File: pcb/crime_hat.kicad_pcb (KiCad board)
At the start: 2 copper layers, 3 parts, among them Q1 2N2222, Q2 FQP27P06

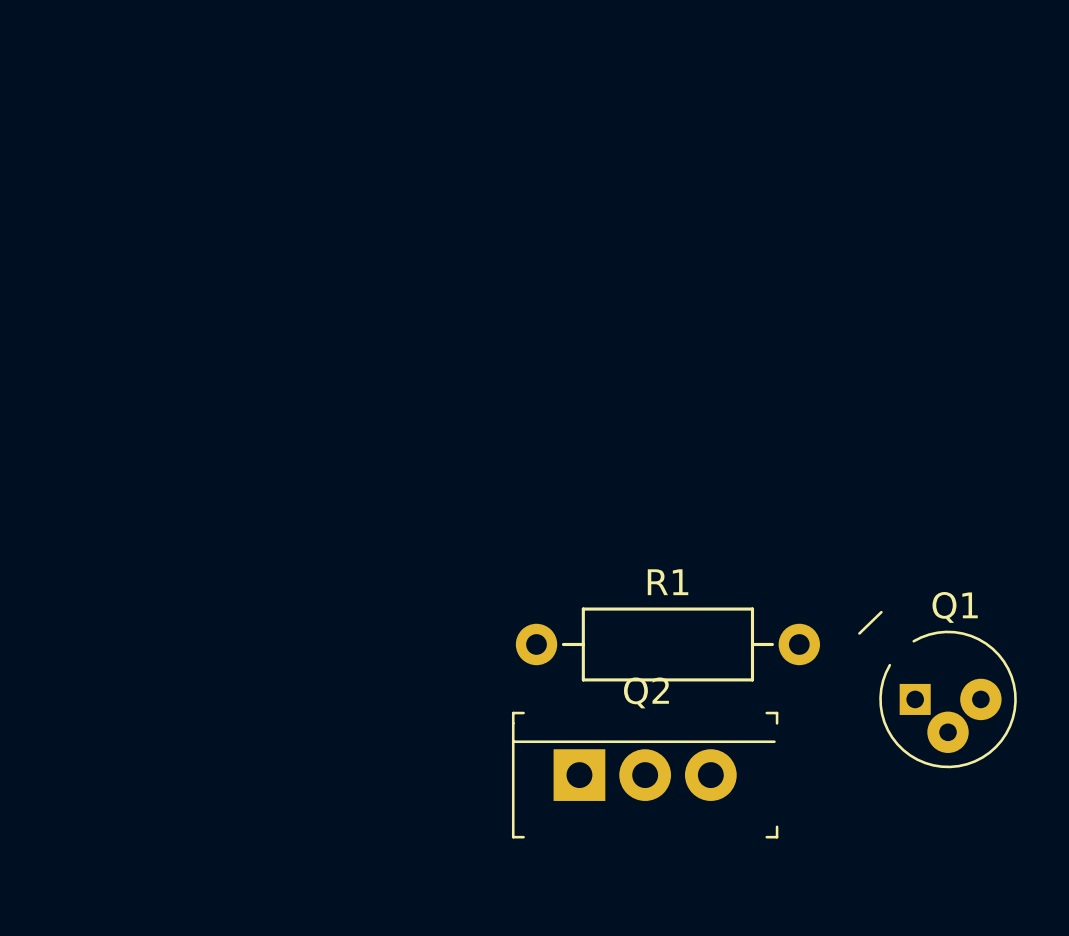
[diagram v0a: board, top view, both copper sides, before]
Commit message: layout
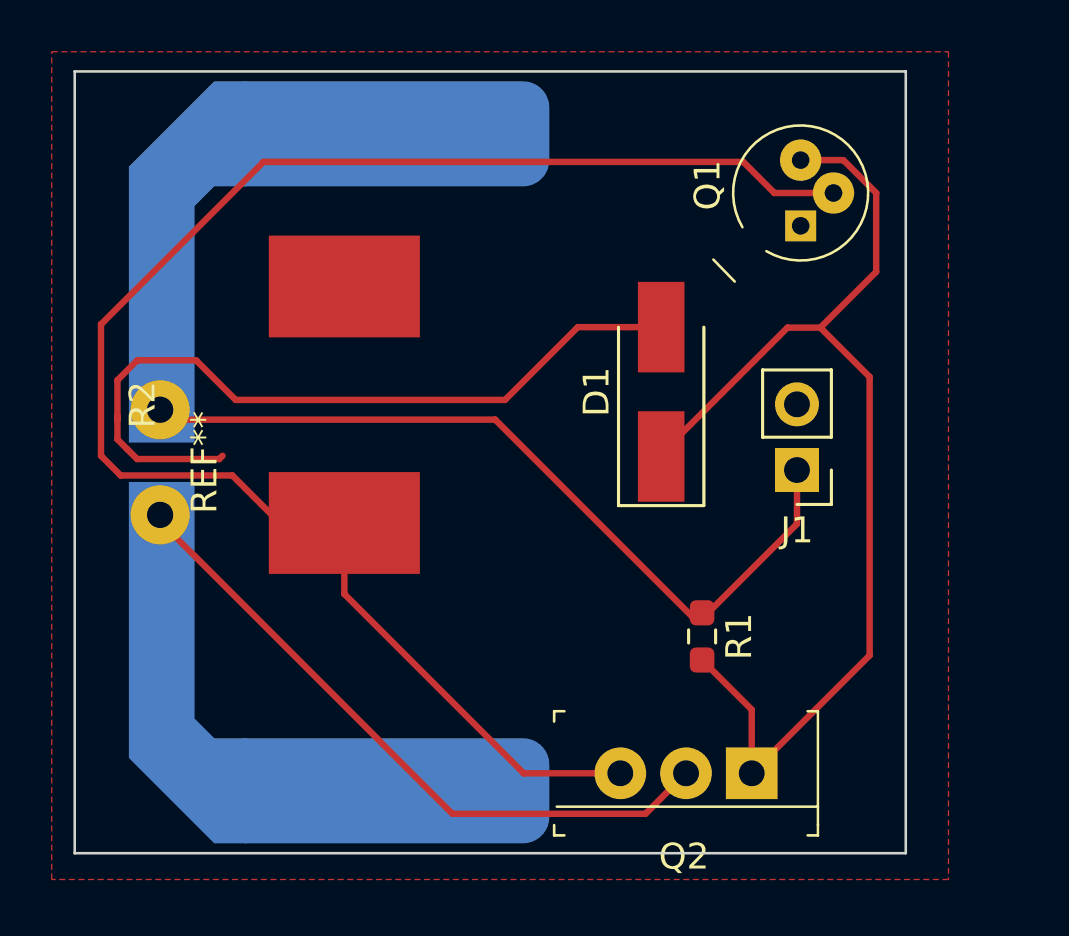
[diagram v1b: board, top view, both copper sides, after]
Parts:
- added D1: 1N4733A, Diode_SMD:D_SMA_Handsoldering, F.Cu at (146.5, 99.0)
- added J1: Conn_01x02_Male, Connector_PinHeader_2.54mm:PinHeader_1x02_P2.54mm_Vertical, F.Cu at (151.8, 102.0)
- added R2: 49.9R, Resistor_SMD:Resistor-WSC000249R90FEB, F.Cu at (134.2, 99.5)
- added REF**: Chanzon_LED, LED_THT:Chanzon_LED, F.Cu at (139.1, 101.7)
- R1: footprint Resistor_THT:R_Axial_DIN0207_L6.3mm_D2.5mm_P10.16mm_Horizontal -> Resistor_SMD:R_0603_1608Metric_Pad0.98x0.95mm_HandSolder
- moved Q1 18.8 mm to (151.9, 92.6), turned to 90 degrees
- moved Q2 6.66 mm to (150.0, 113.8), turned to 180 degrees
- moved R1 6.41 mm to (148.1, 108.5), turned to -90 degrees
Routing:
- net Net-(Q1-Pad2): track 0.00 -> 63.3 mm
- net +9VA: track 0.00 -> 49.7 mm
- net Net-(D2-Pad1): track 0.00 -> 43.8 mm
- net Net-(D1-Pad1): track 0.00 -> 42.9 mm
- net GND: track 0.00 -> 30.0 mm
- added copper zone on F.Cu, net GND
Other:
- board outline added: 32.1 x 30.2 mm
